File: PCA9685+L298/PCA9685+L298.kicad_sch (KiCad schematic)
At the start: 38 parts, among them J1 TERMBLOCK_1X2, Q1 AOD417, U1 PCA9685

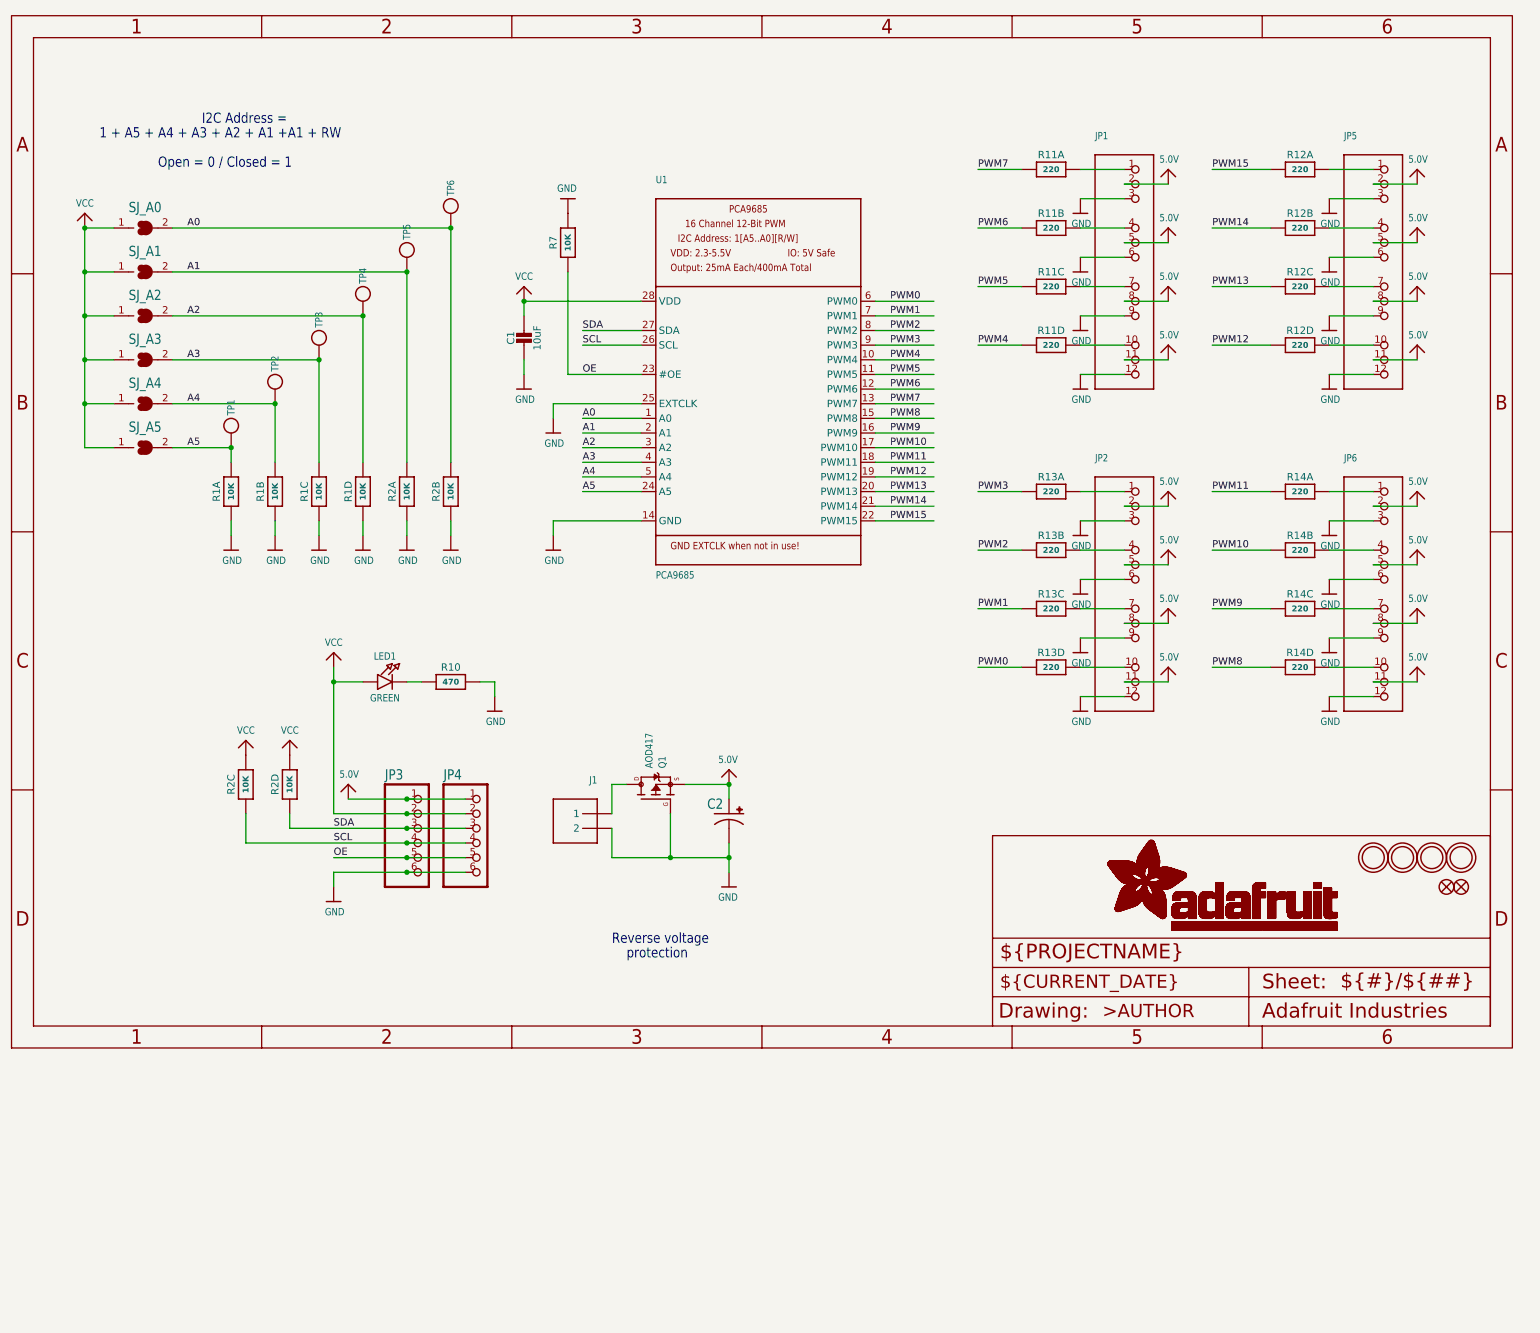
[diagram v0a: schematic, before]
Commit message: .
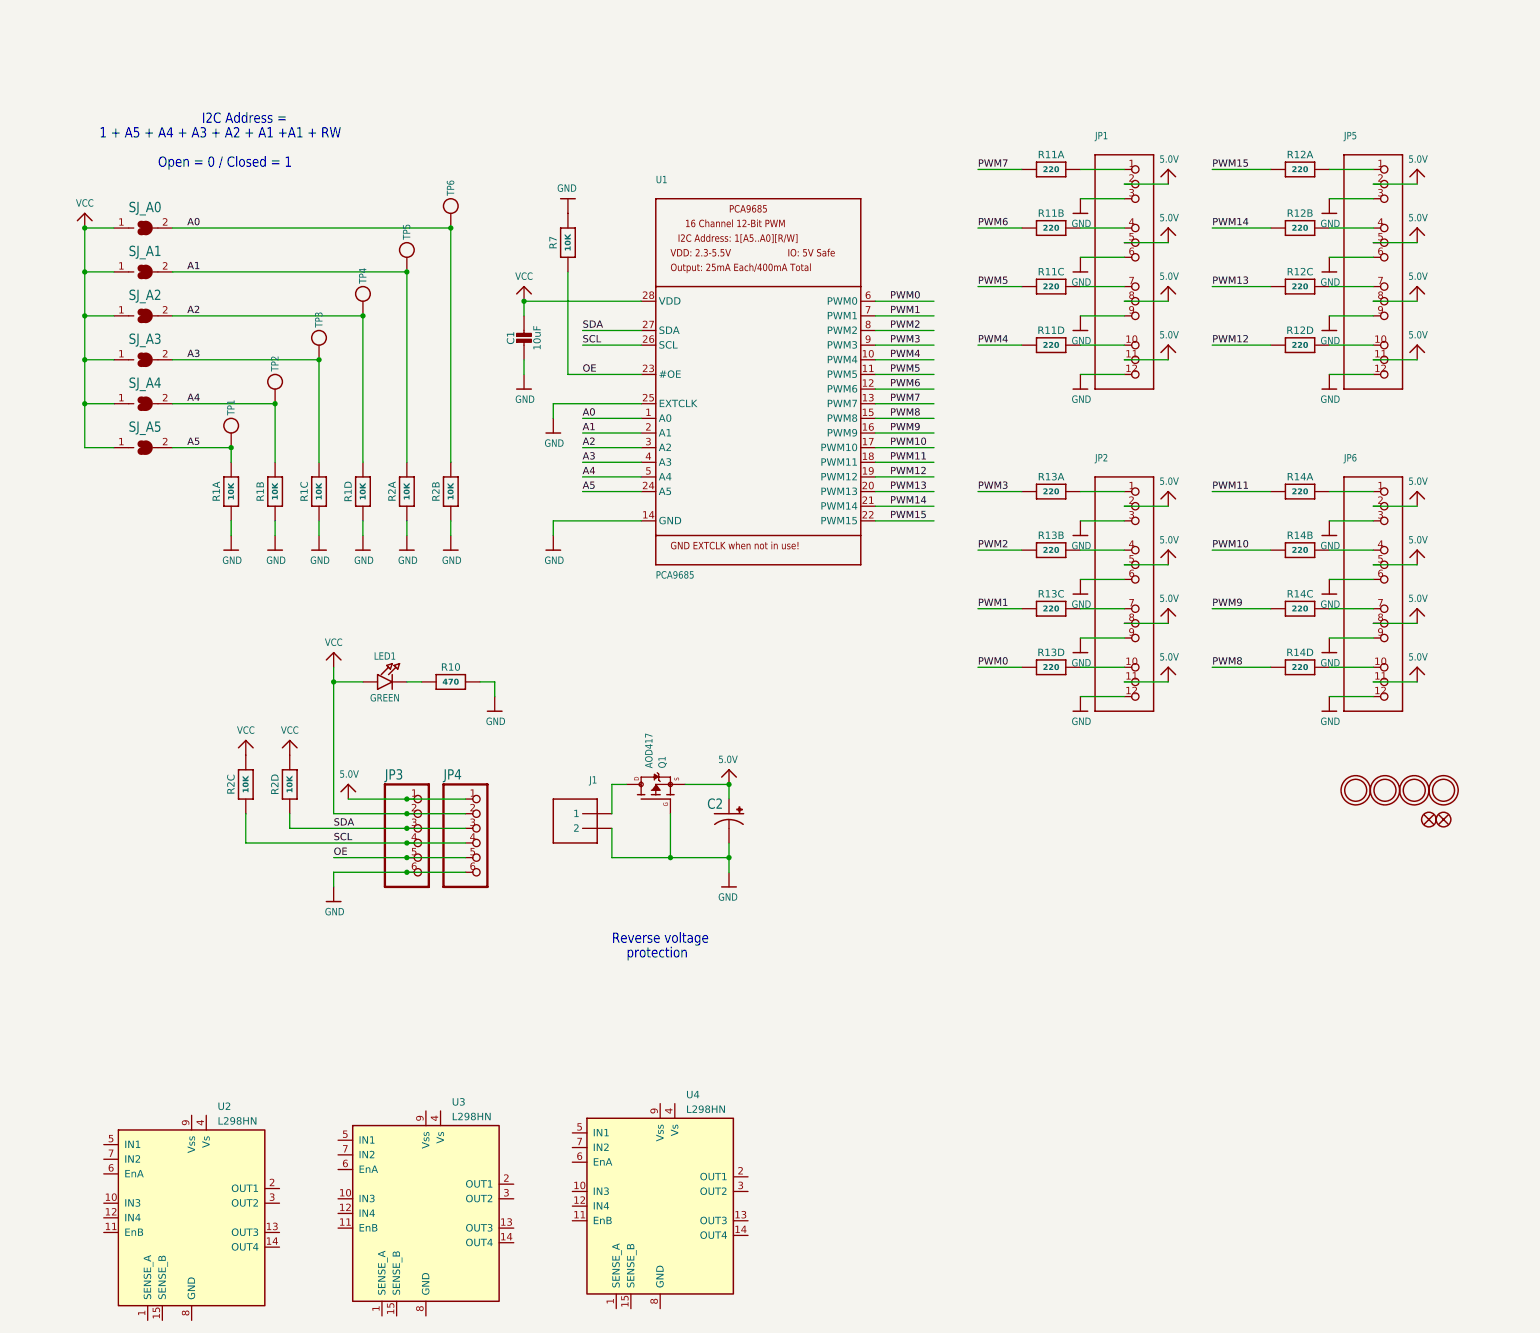
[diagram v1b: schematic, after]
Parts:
- added U2, U3, U4: L298HN, Silicon-Standard:POWERSO20_L298_PAD, symbol Driver_Motor:L298HN
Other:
- company: (none) -> Hasatio
- title: (none) -> PCA9685+L298

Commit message: 18.04.23
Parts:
- removed JP1, JP2, JP5, JP6: HEADER-3X04, Adafruit PCA9685 rev C:3X04, symbol Adafruit PCA9685 rev C-eagle-import:HEADER-3X04
- added C3, C4, C5, C8, C9: 1.0uF, Adafruit PCA9685 rev C:0805-NO, symbol Adafruit PCA9685 rev C-eagle-import:CAP_CERAMIC0805-NOOUTLINE
- added C6, C7: 10uF, Adafruit PCA9685 rev C:0805-NO, symbol Adafruit PCA9685 rev C-eagle-import:CAP_CERAMIC0805-NOOUTLINE
- added D1, D10, D11, D12, D13, D14, D15, D16, D17, D18, D19, D2, D20, D21, D22, D23, D24, D25, D3, D4, D5, D6, D7, D8, D9: M7, Diode_SMD:D_SMA, symbol PCM_Diode_AKL:M7
- added J10, J11, J4, J5, J7, J8: TERMBLOCK_1X2, Adafruit PCA9685 rev C:TERMBLOCK_1X2-3.5MM, symbol Adafruit PCA9685 rev C-eagle-import:TERMBLOCK_1X2
- added J13, J3, J6, J9: Conn_01x04, Connector_PinHeader_2.54mm:PinHeader_1x04_P2.54mm_Vertical, symbol Connector_Generic:Conn_01x04
- added J7 (x2): QWIIC_RIGHT_ANGLE, Connectors:1X04_1MM_RA_STRESSRELIEF, symbol SparkFun ESP32 Thing Plus C-eagle-import:QWIIC_CONNECTORJS-1MM
- added JP1 (x8): JUMPER-SMT_2_NC_TRACE_SILK, OLIMEX_Jumpers-FP:SJ_Closed, symbol SparkFun ESP32 Thing Plus C-eagle-import:JUMPER-SMT_2_NC_TRACE_SILK
- added LED2: RED, Adafruit PCA9685 rev C:CHIPLED_0805_NOOUTLINE, symbol Adafruit PCA9685 rev C-eagle-import:LED0805_NOOUTLINE
- added R5: 470, Adafruit PCA9685 rev C:_0805MP, symbol Adafruit PCA9685 rev C-eagle-import:RESISTOR_0805MP
- added U5, U6, U7: ADS1115IDGS, Package_SO:TSSOP-10_3x3mm_P0.5mm, symbol Analog_ADC:ADS1115IDGS
- added U8: L7805, PCM_Package_TO_SOT_SMD_AKL:TO-252-3_TabPin2, symbol Regulator_Linear:L7805
- renumbered R7 to R3, R10 to R4
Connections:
- net 5.0V: now also C1.1, SJ_A0.1, SJ_A1.1, SJ_A2.1, SJ_A3.1, SJ_A4.1, SJ_A5.1, U1.28 (VDD), U2.9 (Vss), U3.9 (Vss), U4.9 (Vss), C7.1, C9.1, D1.2 (A), JP1.2, JP1.2, JP1.2, JP1.2, JP1.2, JP1.2, JP1.2, U8.3 (OUT); no longer C2.+, Q1.2 (S)
- net GND: now also U2.1 (SENSE_A), U2.15 (SENSE_B), U2.8 (GND), U3.1 (SENSE_A), U3.15 (SENSE_B), U3.8 (GND), U4.1 (SENSE_A), U4.15 (SENSE_B), U4.8 (GND), C3.2, C4.2, C5.2, C6.2, C7.2, C8.2, C9.2, D11.2 (A), D13.2 (A), D15.2 (A), D17.2 (A), D19.2 (A), D21.2 (A), D23.2 (A), D25.2 (A), D3.2 (A), D5.2 (A), D7.2 (A), D9.2 (A), J7.1, J7.1, R5.2, U5.1 (ADDR), U5.3 (GND), U6.3 (GND), U7.3 (GND), U8.2 (GND)
- net SCL: now also J7.4, J7.4, U5.10 (SCL), U6.10 (SCL), U7.1 (ADDR), U7.9 (SDA)
- net SDA: now also J7.3, J7.3, U5.9 (SDA), U6.9 (SDA), U7.10 (SCL)
- net VCC: now also C2.+, Q1.2 (S), U2.4 (Vs), U3.4 (Vs), U4.4 (Vs), C6.1, C8.1, D1.1 (K), D10.1 (K), D12.1 (K), D14.1 (K), D16.1 (K), D18.1 (K), D2.1 (K), D20.1 (K), D22.1 (K), D24.1 (K), D4.1 (K), D6.1 (K), D8.1 (K), JP1.2, U8.1 (IN); no longer C1.1, LED1.A, SJ_A0.1, SJ_A1.1, SJ_A2.1, SJ_A3.1, SJ_A4.1, SJ_A5.1, U1.28 (VDD)
- net at R12.7 (2): now also J13.3 (Pin_3)
- net P11: now reaches R14.8 (2)
- net P11: now also U4.5 (IN1)
- net P8: now reaches R14.5 (2)
- net P8: now also U4.12 (IN4)
- net P10: now reaches R14.7 (2)
- net P10: now also U4.7 (IN2)
- net P9: now reaches R14.6 (2)
- net P9: now also U4.10 (IN3)
- net P7: now reaches R11.8 (2)
- net P7: now also U3.5 (IN1)
- net P5: now reaches R11.6 (2)
- net P5: now also U3.10 (IN3)
- net P3: now reaches R13.8 (2)
- net P3: now also U2.5 (IN1)
- net P0: now reaches R13.5 (2)
- net P0: now also U2.12 (IN4)
- net P2: now reaches R13.7 (2)
- net P2: now also U2.7 (IN2)
- net P1: now reaches R13.6 (2)
- net P1: now also U2.10 (IN3)
- net P4: now reaches R11.5 (2)
- net P4: now also U3.12 (IN4)
- net at R12.6 (2): now also J13.2 (Pin_2)
- net at R12.8 (2): now also J13.4 (Pin_4)
- net at R12.5 (2): now also J13.1 (Pin_1)
- net at U3.11 (EnB): now also JP1.1
- net at U3.13 (OUT3): now also D14.2 (A), D15.1 (K), J8.1
- net at U3.14 (OUT4): now also D16.2 (A), D17.1 (K), J8.2
- net at U3.2 (OUT1): now also D10.2 (A), D11.1 (K), J7.1
- net at U3.3 (OUT2): now also D12.2 (A), D13.1 (K), J7.2
- net at U3.6 (EnA): now also JP1.1
- net P6: now reaches U3.7 (IN2)
- net P6: now also R11.7 (2)
- net at U2.11 (EnB): now also JP1.1
- net at U2.13 (OUT3): now also D6.2 (A), D7.1 (K), J5.1
- net at U2.14 (OUT4): now also D8.2 (A), D9.1 (K), J5.2
- net at U2.2 (OUT1): now also D2.2 (A), D3.1 (K), J4.1
- net at U2.3 (OUT2): now also D4.2 (A), D5.1 (K), J4.2
- net at U2.6 (EnA): now also JP1.1
- net at U4.11 (EnB): now also JP1.1
- net at U4.13 (OUT3): now also D22.2 (A), D23.1 (K), J11.1
- net at U4.14 (OUT4): now also D24.2 (A), D25.1 (K), J11.2
- net at U4.2 (OUT1): now also D18.2 (A), D19.1 (K), J10.1
- net at U4.3 (OUT2): now also D20.2 (A), D21.1 (K), J10.2
- net at U4.6 (EnA): now also JP1.1
- new net: J9.1 (Pin_1), U7.4 (AIN0)
- new net: J9.2 (Pin_2), U7.5 (AIN1)
- new net: J9.3 (Pin_3), U7.6 (AIN2)
- new net: J9.4 (Pin_4), U7.7 (AIN3)
- new net: JP1.1, LED2.A
- new net: LED2.C, R5.1
- new net: J6.1 (Pin_1), U6.4 (AIN0)
- new net: J6.2 (Pin_2), U6.5 (AIN1)
- new net: J6.3 (Pin_3), U6.6 (AIN2)
- new net: J6.4 (Pin_4), U6.7 (AIN3)
- new net: J3.1 (Pin_1), U5.4 (AIN0)
- new net: J3.2 (Pin_2), U5.5 (AIN1)
- new net: J3.3 (Pin_3), U5.6 (AIN2)
- new net: J3.4 (Pin_4), U5.7 (AIN3)
- new net: JP1.1, LED1.A
- new net 3.3V: C3.1, C4.1, C5.1, J7.2, J7.2, U5.8 (VDD), U6.1 (ADDR), U6.8 (VDD), U7.8 (VDD)
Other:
- note added: "Analog"
- note added: "Jumper"
- note added: "L298"
- note added: "PCA9685"
- note added: "Qwiic"
- note added: "Regulator"
- moved on the sheet: C1, C2, J1, JP3, JP4, LED1, Q1, R11A, R11B, R11C, R11D, R12A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
